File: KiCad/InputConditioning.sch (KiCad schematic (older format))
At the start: 30 parts

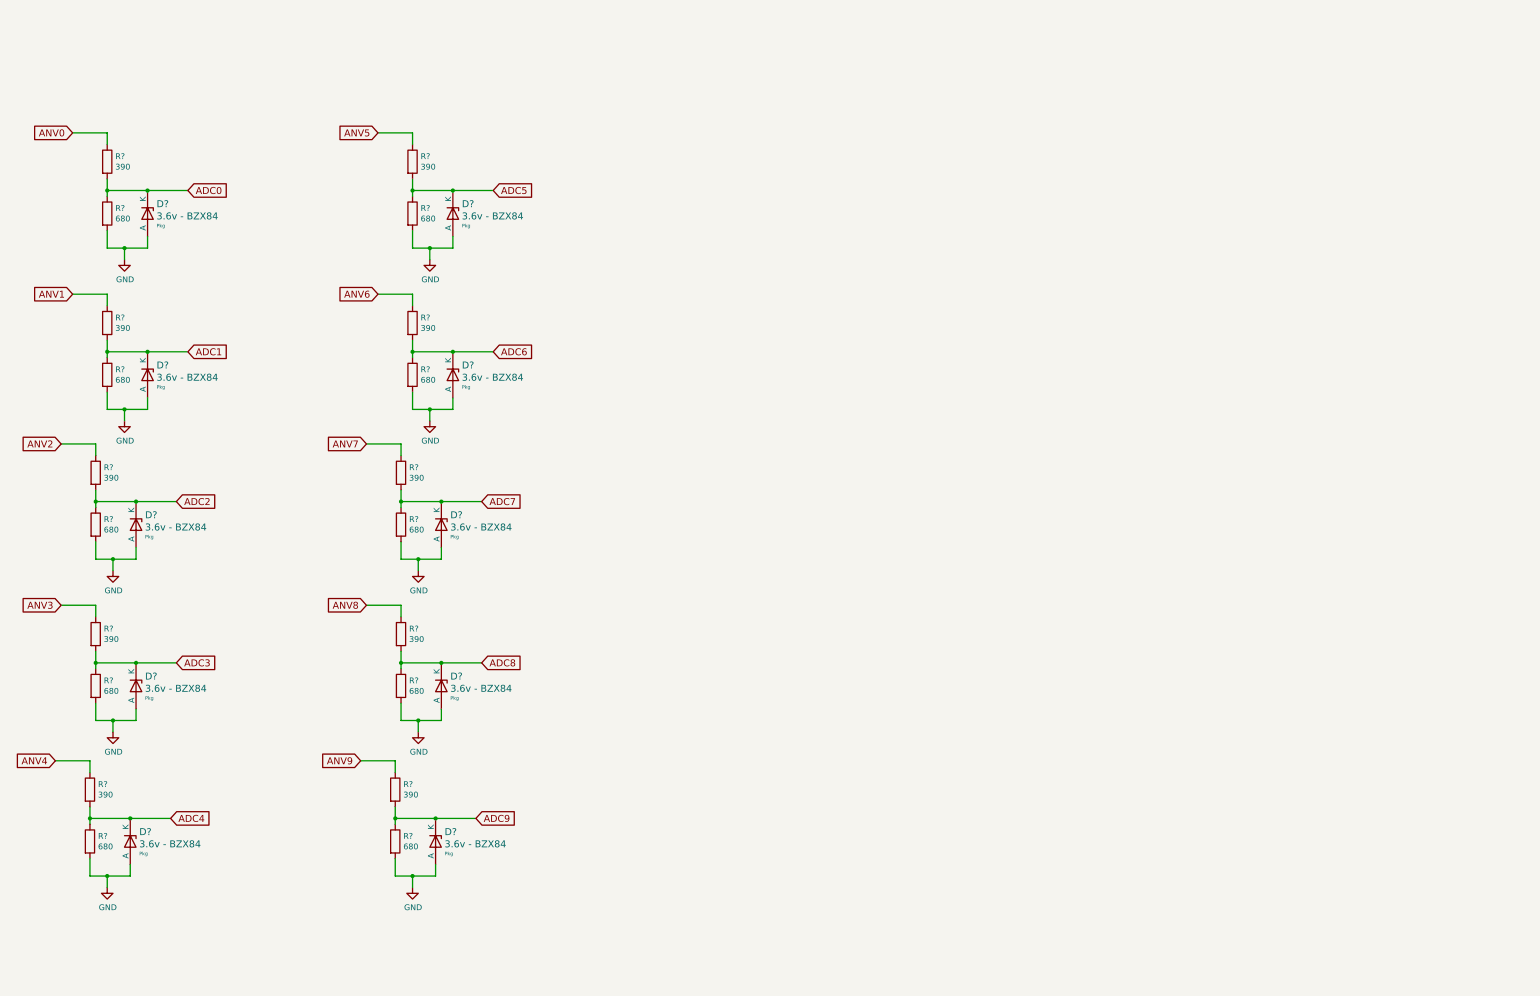
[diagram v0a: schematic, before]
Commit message: Routine
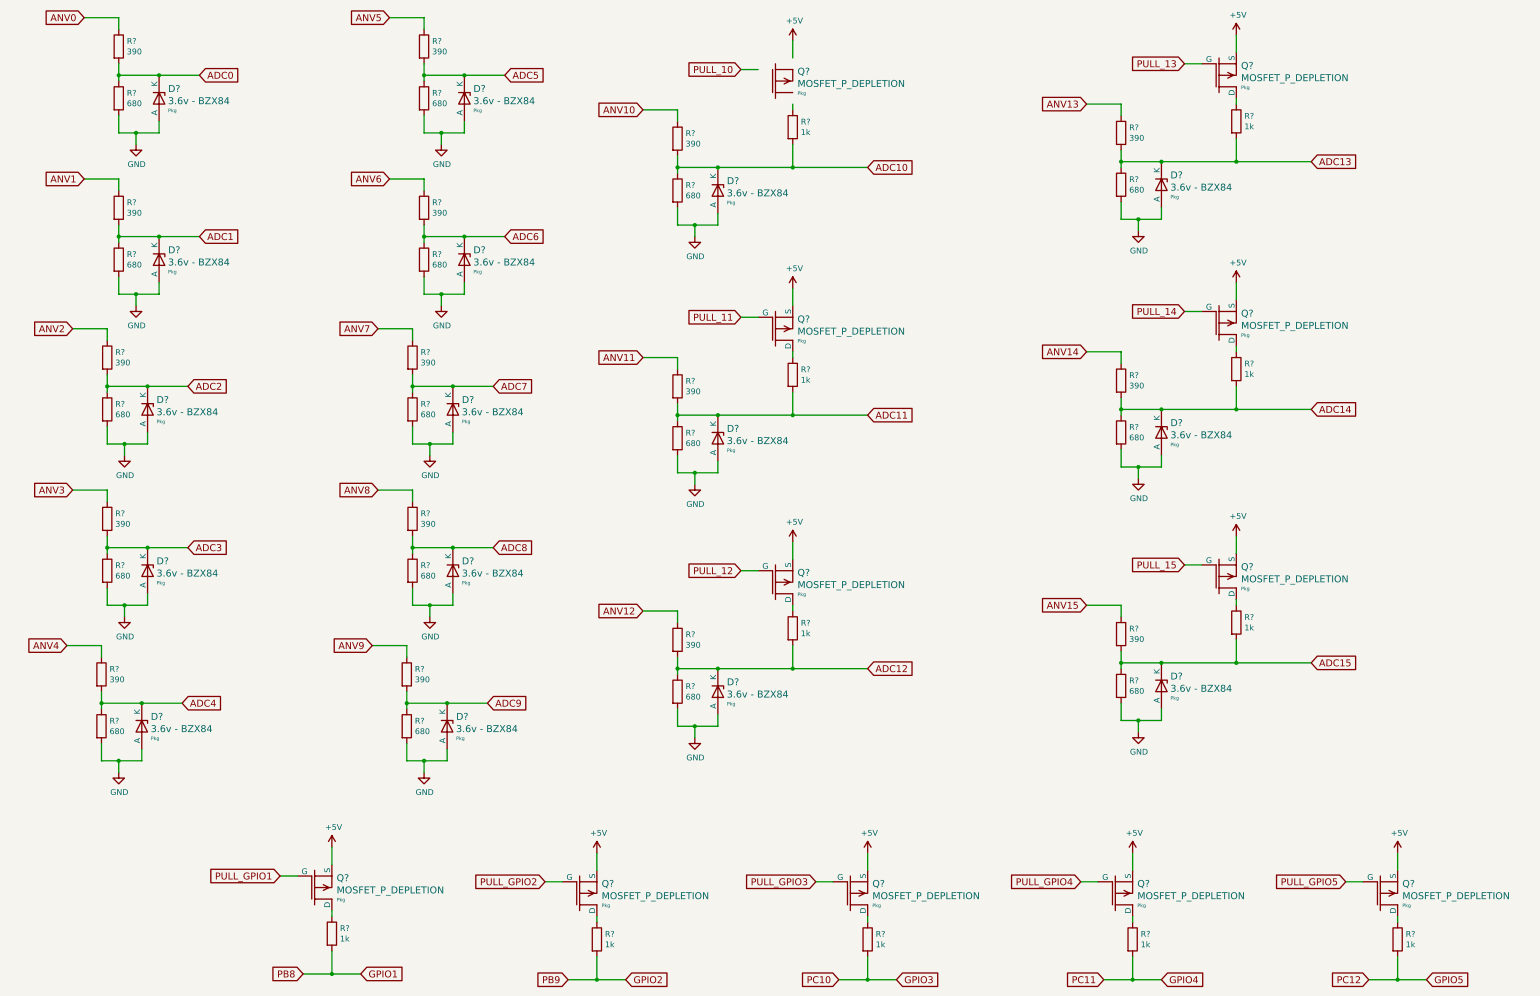
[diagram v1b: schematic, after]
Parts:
- added D? (x6): 3.6v - BZX84, Pkg, symbol DIODE_ZENER
- added Q? (x11): MOSFET_P_DEPLETION, Pkg, symbol MOSFET_P_DEPLETION
- added R? (x6): 390, symbol R
- added R? (x6): 680, symbol R
- added R? (x11): 1k, symbol R
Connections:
- net GND: now also D?.A, D?.A, D?.A, D?.A, D?.A, D?.A, R?.2, R?.2, R?.2, R?.2, R?.2, R?.2
- new net: Q?.D, R?.1 (x10)
- new net +5V: Q?.S, Q?.S, Q?.S, Q?.S, Q?.S, Q?.S, Q?.S, Q?.S, Q?.S, Q?.S
- new net ADC10: D?.K, R?.1, R?.2, R?.2
- new net ADC11: D?.K, R?.1, R?.2, R?.2
- new net ADC12: D?.K, R?.1, R?.2, R?.2
- new net ADC13: D?.K, R?.1, R?.2, R?.2
- new net ADC14: D?.K, R?.1, R?.2, R?.2
- new net ADC15: D?.K, R?.1, R?.2, R?.2
- new net ANV10: R?.1
- new net ANV11: R?.1
- new net ANV12: R?.1
- new net ANV13: R?.1
- new net ANV14: R?.1
- new net ANV15: R?.1
- new net GPIO1: R?.2
- new net GPIO2: R?.2
- new net GPIO3: R?.2
- new net GPIO4: R?.2
- new net GPIO5: R?.2
- new net PULL_11: Q?.G
- new net PULL_12: Q?.G
- new net PULL_13: Q?.G
- new net PULL_14: Q?.G
- new net PULL_15: Q?.G
- new net PULL_GPIO1: Q?.G
- new net PULL_GPIO2: Q?.G
- new net PULL_GPIO3: Q?.G
- new net PULL_GPIO4: Q?.G
- new net PULL_GPIO5: Q?.G
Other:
- moved on the sheet: D?, R?
